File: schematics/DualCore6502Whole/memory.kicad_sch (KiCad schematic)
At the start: 6 parts, among them U10 28C256, U8 74HC86, U9 62256

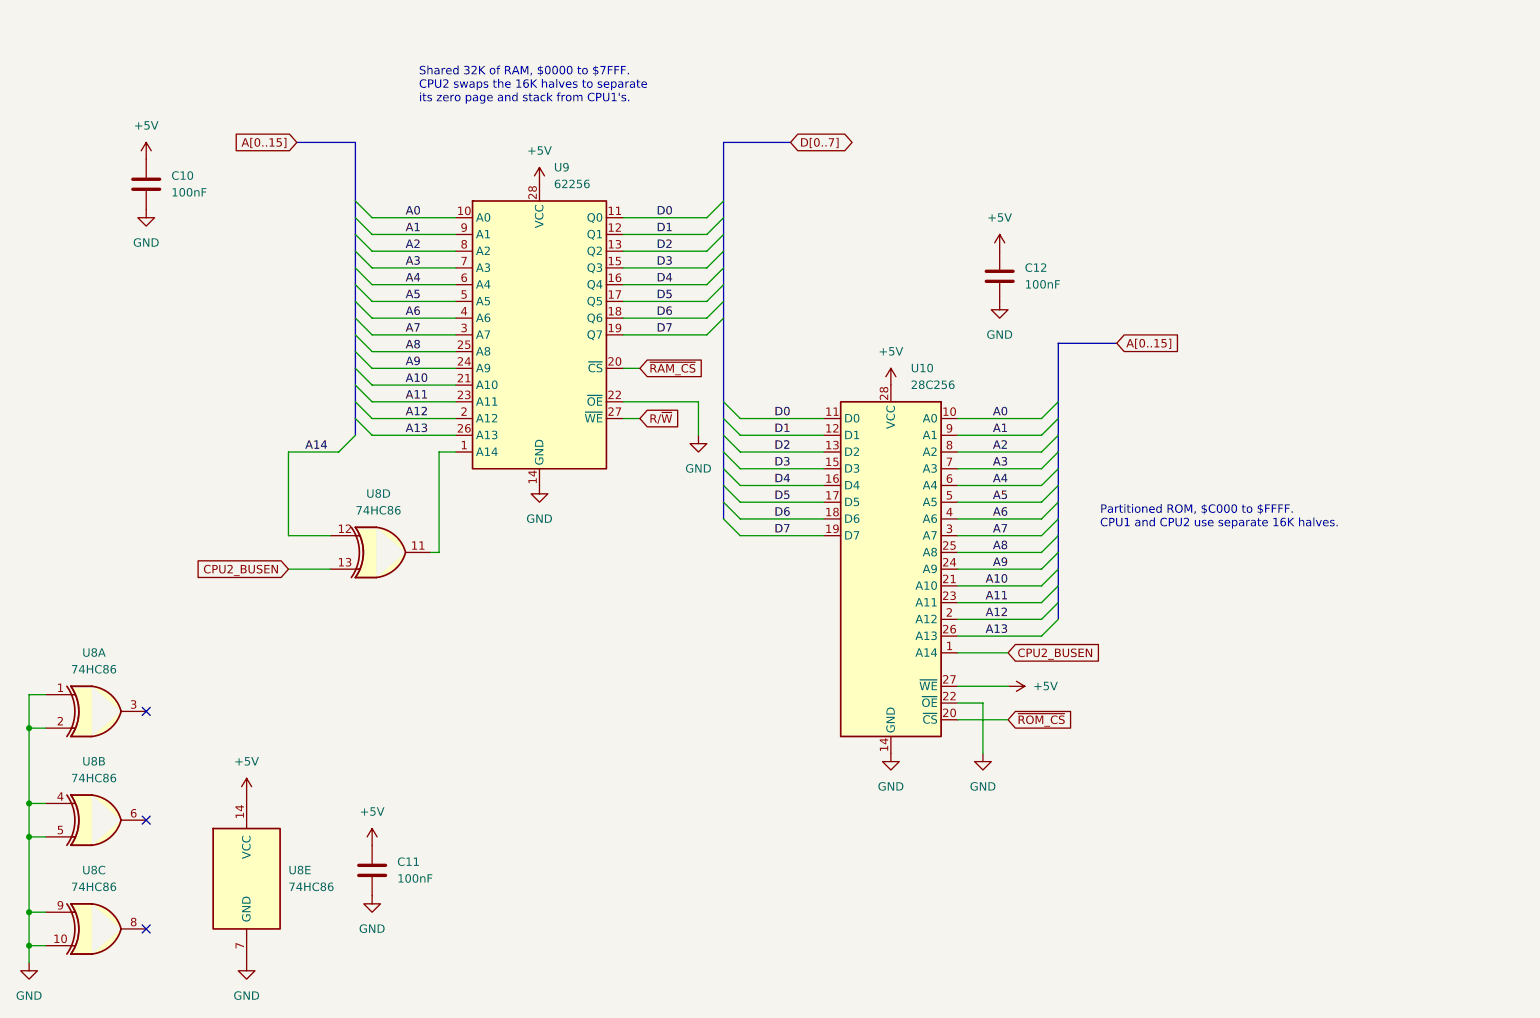
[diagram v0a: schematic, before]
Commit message: Update the schematic
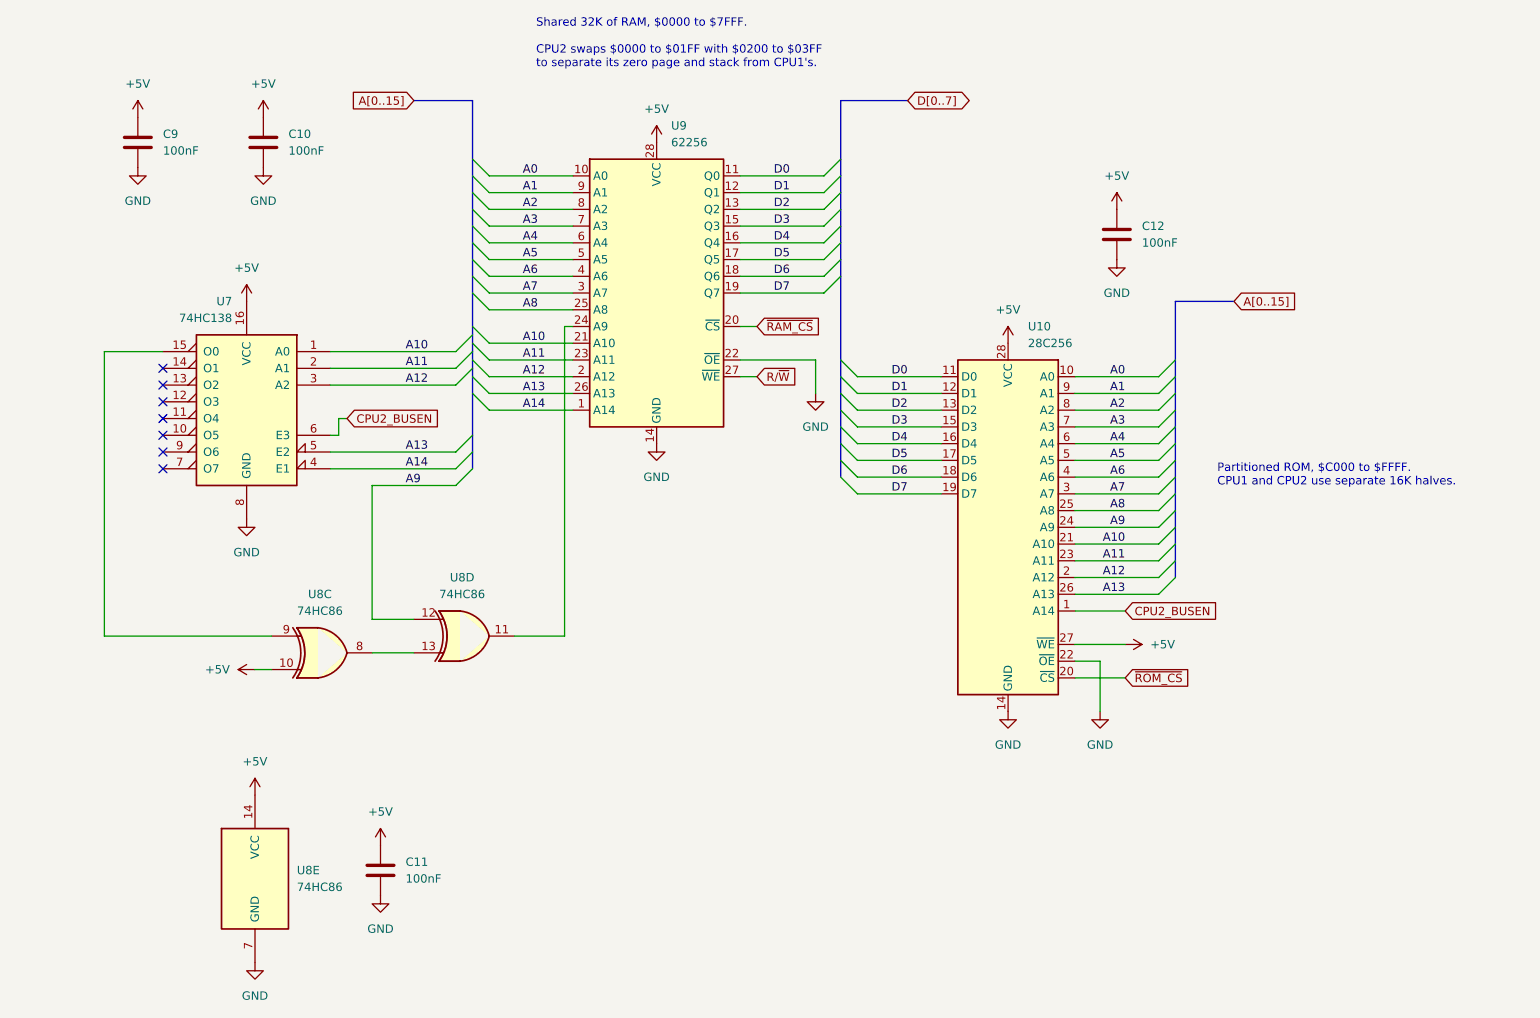
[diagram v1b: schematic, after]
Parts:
- removed unit 2 of U8
- removed unit 1 of U8
- added C9: 100nF, Capacitor_THT:C_Disc_D5.0mm_W2.5mm_P5.00mm, symbol Device:C
- added U7: 74HC138, Package_DIP:DIP-16_W7.62mm, symbol 74xx:74LS138
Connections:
- net +5V: now also U8.10, C9.1, U7.16 (VCC)
- net A10: now also U7.1 (A0)
- net A11: now also U7.2 (A1)
- net A12: now also U7.3 (A2)
- net A13: now also U7.5 (E2)
- net A14: now also U9.1 (A14), U7.4 (E1); no longer U8.12
- net A9: now also U8.12; no longer U9.24 (A9)
- net CPU2_BUSEN: now also U7.6 (E3); no longer U8.13
- net GND: now also C9.2, U7.8 (GND); no longer U8.10, U8.9
- net at U8.11: now also U9.24 (A9); no longer U9.1 (A14)
- net at U8.8: now also U8.13
- new net: U7.15 (O0), U8.9
- no-connect marks 3 -> 7
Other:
- note added: "Shared 32K of RAM, $0000 to $7FFF. CPU2 swaps $0000 to $01FF with $0200 to $03FF to separate its zero page and stack from CPU1's."
- note removed: "Shared 32K of RAM, $0000 to $7FFF. CPU2 swaps the 16K halves to separate its zero page and stack from CPU1's."
- title: (none) -> Dual Core 65C02 Computer
- moved on the sheet: C10, C11, C12, U10, U8C, U8D, U8E, U9
